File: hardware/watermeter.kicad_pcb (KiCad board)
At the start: 2 copper layers, 80 x 40 mm, 46 parts, among them J1 TC2030, J2 EXT, J3 flow_meter, J4 PT1000-1, J5 PT1000-2, J6 24V_Power, SW1 Reboot, U1 ESP32-C6-MINI-1, U2 TLV2462AID, U3 K7805-500R3, U4 LM3671MFX-3.3/NOPB

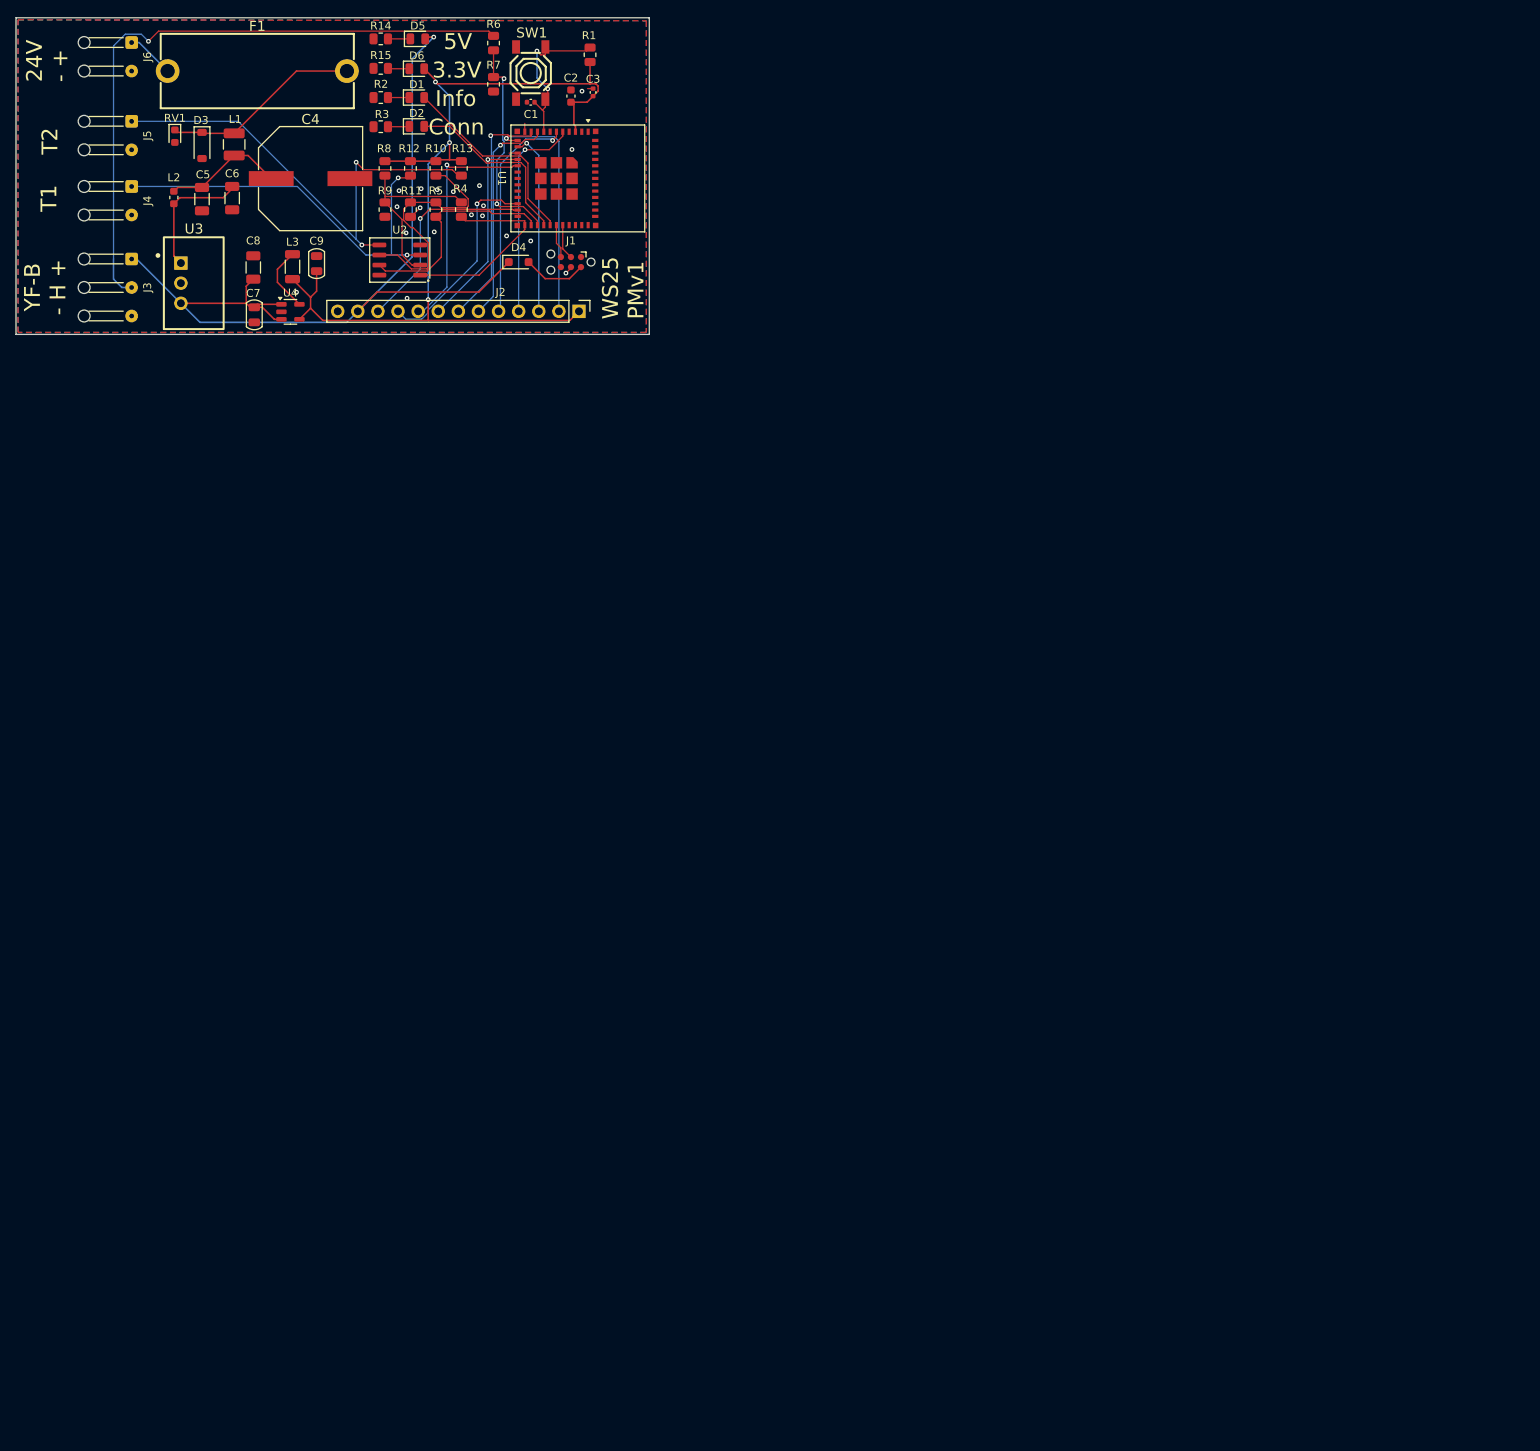
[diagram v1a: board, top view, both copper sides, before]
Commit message: Release hardware design v1.0 for manufacturing
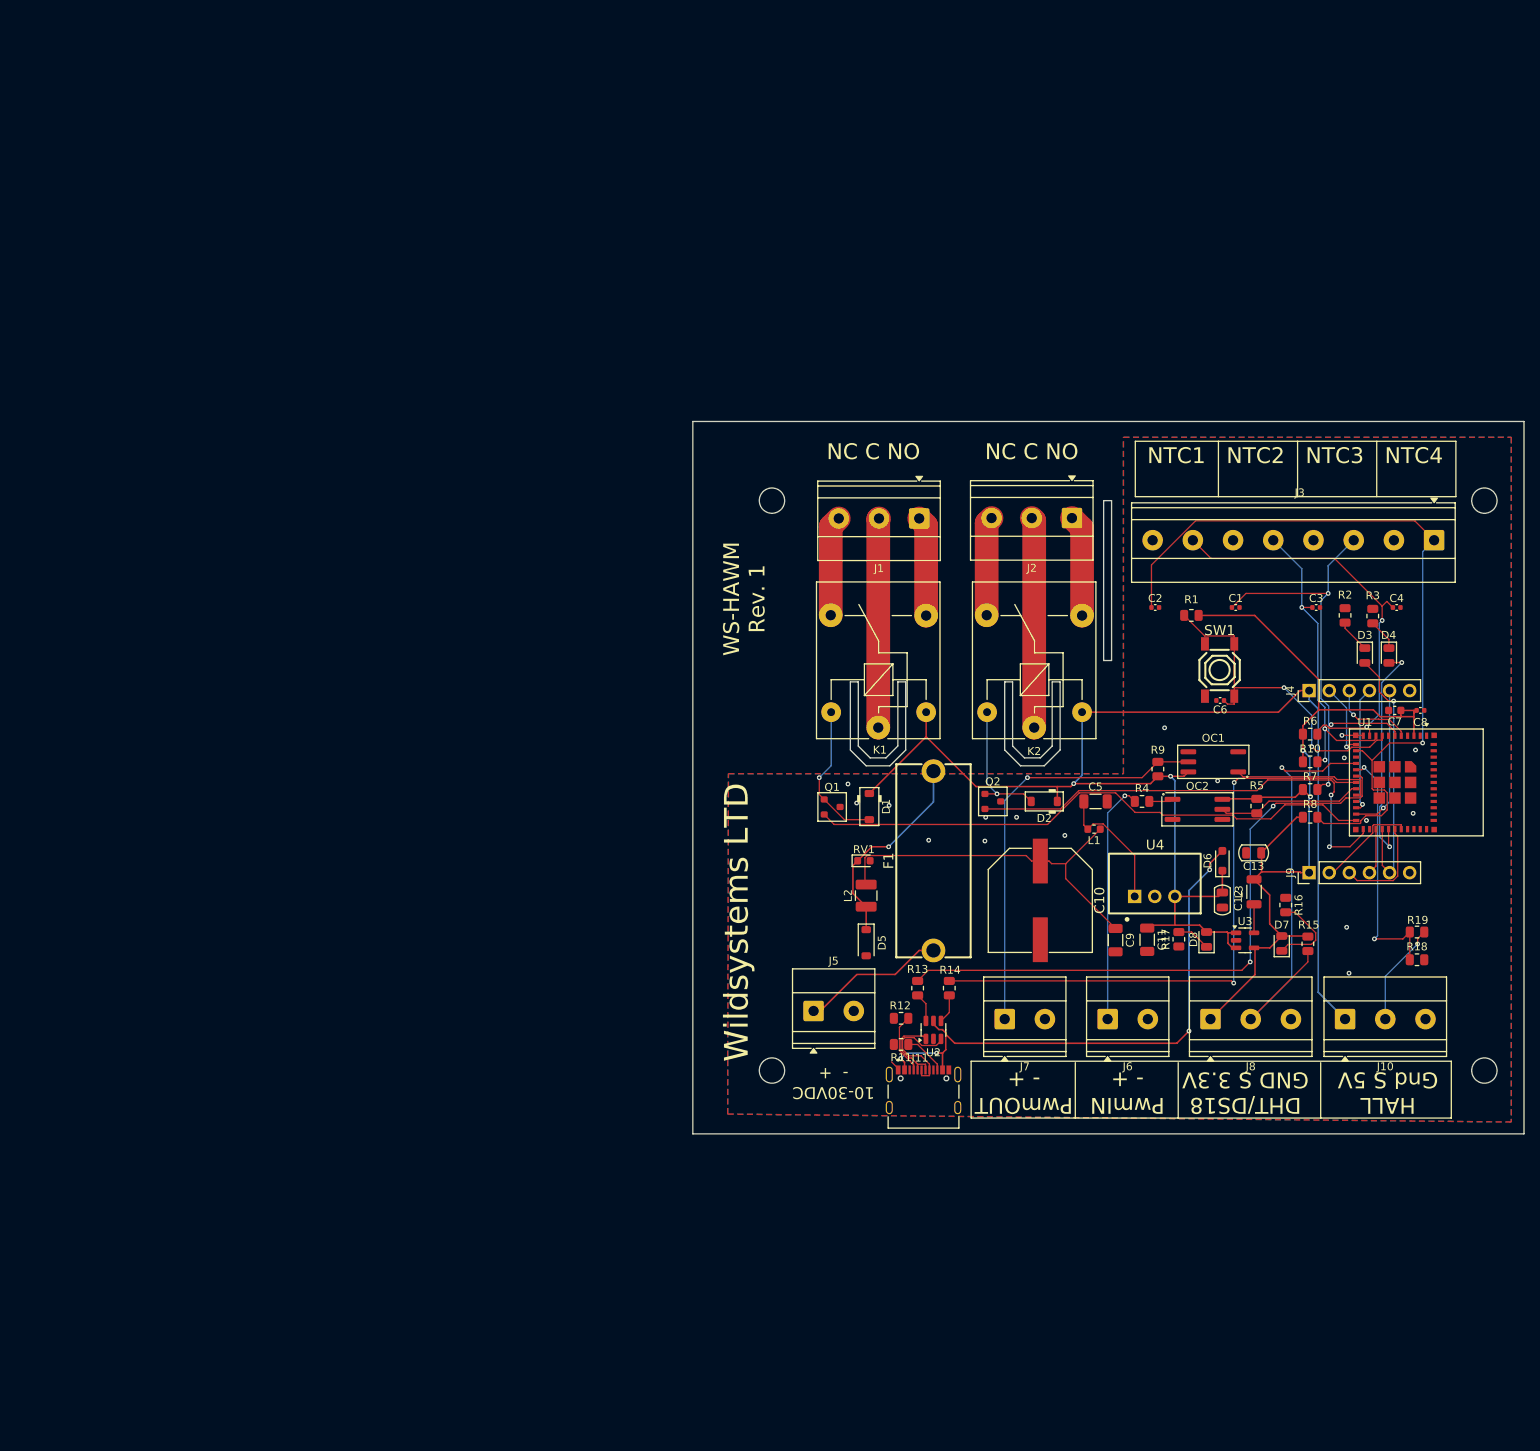
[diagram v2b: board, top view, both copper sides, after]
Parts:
- added C10: 680uF/50V, MyFootprints:CAP-SMD_BD12.5-L13.0-W13.0-LS14.4-FD, F.Cu at (129.4, 111.5)
- added C11: 22uF/10V, Capacitor_SMD:C_1206_3216Metric, F.Cu at (142.9, 116.5)
- added C12: 4.7uF/10V, PCM_Capacitor_SMD_AKL:C_0805_2012Metric, F.Cu at (152.4, 111.5)
- added C13: 10uF, PCM_Capacitor_SMD_AKL:C_0805_2012Metric, F.Cu at (156.3, 105.5)
- added D7: KT-0805G, LED_SMD:LED_0805_2012Metric, F.Cu at (159.9, 116.9)
- added D8: KT-0805G, LED_SMD:LED_0805_2012Metric, F.Cu at (150.4, 116.4)
- added H1: MountingHole, MountingHole:MountingHole_3.2mm_M3_ISO7380, F.Cu at (95.5, 61.0)
- added H2: MountingHole, MountingHole:MountingHole_3.2mm_M3_ISO7380, F.Cu at (185.5, 61.0)
- added H3: MountingHole, MountingHole:MountingHole_3.2mm_M3_ISO7380, F.Cu at (95.5, 133.0)
- added H4: MountingHole, MountingHole:MountingHole_3.2mm_M3_ISO7380, F.Cu at (185.5, 133.0)
- added J10: flow_meter, TerminalBlock_Phoenix:TerminalBlock_Phoenix_MKDS-1,5-3-5.08_1x03_P5.08mm_Horizontal, F.Cu at (167.9, 126.5)
- added J11: USB-TYPE-C-31-M-12, MyFootprints:USB-HRO_TYPE-C-31-M-12, F.Cu at (114.6, 137.7)
- added J7: PWM_OUT, TerminalBlock_Phoenix:TerminalBlock_Phoenix_MKDS-1,5-2-5.08_1x02_P5.08mm_Horizontal, F.Cu at (124.9, 126.5)
- added J8: DHT21, TerminalBlock_Phoenix:TerminalBlock_Phoenix_MKDS-1,5-3-5.08_1x03_P5.08mm_Horizontal, F.Cu at (150.9, 126.5)
- added J9: Conn_01x06_Shielded, Connector_PinHeader_2.54mm:PinHeader_1x06_P2.54mm_Vertical, F.Cu at (163.4, 108.0)
- added K1: SRD-05VDC-SL-C, Relay_THT:Relay_SPDT_SANYOU_SRD_Series_Form_C, F.Cu at (108.9, 89.7)
- added K2: SRD-05VDC-SL-C, Relay_THT:Relay_SPDT_SANYOU_SRD_Series_Form_C, F.Cu at (128.6, 89.7)
- added OC1: TLP2361, PCM_Package_SO_AKL:SO-5_4.4x3.6mm_P1.27mm, F.Cu at (151.2, 94.0)
- added OC2: TLP2361, PCM_Package_SO_AKL:SO-5_4.4x3.6mm_P1.27mm, F.Cu at (149.2, 100.0)
- added Q1: NPN, PCM_Package_TO_SOT_SMD_AKL:SOT-23, F.Cu at (103.1, 99.7)
- added Q2: NPN, PCM_Package_TO_SOT_SMD_AKL:SOT-23, F.Cu at (123.4, 99.0)
- added R16: 20R, Resistor_SMD:R_0805_2012Metric, F.Cu at (160.4, 112.1)
- added R17: 20R, Resistor_SMD:R_0805_2012Metric, F.Cu at (146.9, 116.4)
- added R18: 2k, Resistor_SMD:R_0805_2012Metric, F.Cu at (177.0, 119.0)
- added R19: 1k, Resistor_SMD:R_0805_2012Metric, F.Cu at (177.0, 115.5)
- C1: value 1uF -> 0.1uF
- C2: value 22uF -> 0.1uF; footprint Capacitor_SMD:C_0603_1608Metric -> Capacitor_SMD:C_0402_1005Metric
- C4: value 680uF/50V -> 0.1uF; footprint MyFootprints:CAP-SMD_BD12.5-L13.0-W13.0-LS14.4-FD -> Capacitor_SMD:C_0402_1005Metric
- C5: value 4.7uF/63V -> 10uF/50V
- C6: value 10uF/50V -> 1uF; footprint Capacitor_SMD:C_1206_3216Metric -> Capacitor_SMD:C_0402_1005Metric
- C7: value 4.7uF/10V -> 22uF; footprint PCM_Capacitor_SMD_AKL:C_0805_2012Metric -> Capacitor_SMD:C_0603_1608Metric
- C8: value 22uF/10V -> 0.1uF; footprint Capacitor_SMD:C_1206_3216Metric -> Capacitor_SMD:C_0402_1005Metric
- C9: value 10uF -> 4.7uF/63V; footprint PCM_Capacitor_SMD_AKL:C_0805_2012Metric -> Capacitor_SMD:C_1206_3216Metric
- D1: value KT-0805G -> 1N4148W; footprint LED_SMD:LED_0805_2012Metric -> PCM_Diode_SMD_AKL:D_SOD-123
- D2: value KT-0805B -> 1N4148W; footprint Diode_SMD:D_0805_2012Metric -> PCM_Diode_SMD_AKL:D_SOD-123
- D3: value BAT46W -> KT-0805B; footprint Diode_SMD:D_SOD-123 -> Diode_SMD:D_0805_2012Metric
- D4: value 1N5819 -> KT-0805G; footprint Diode_SMD:D_SOD-323_HandSoldering -> LED_SMD:LED_0805_2012Metric
- D5: value KT-0805G -> BAT46W; footprint LED_SMD:LED_0805_2012Metric -> Diode_SMD:D_SOD-123
- D6: value KT-0805G -> 1N5819; footprint LED_SMD:LED_0805_2012Metric -> Diode_SMD:D_SOD-323_HandSoldering
- J1: value TC2030 -> Screw_Terminal_01x03; footprint Connector:Tag-Connect_TC2030-IDC-NL_2x03_P1.27mm_Vertical -> TerminalBlock_Phoenix:TerminalBlock_Phoenix_MKDS-1,5-3-5.08_1x03_P5.08mm_Horizontal
- J2: value EXT -> Screw_Terminal_01x03; footprint Connector_PinHeader_2.54mm:PinHeader_1x13_P2.54mm_Vertical -> TerminalBlock_Phoenix:TerminalBlock_Phoenix_MKDS-1,5-3-5.08_1x03_P5.08mm_Horizontal
- J3: value flow_meter -> Conn_01x08_Pin; footprint Connector_Wire:SolderWire-0.1sqmm_1x03_P3.6mm_D0.4mm_OD1mm_Relief -> TerminalBlock_Phoenix:TerminalBlock_Phoenix_MKDS-1,5-8-5.08_1x08_P5.08mm_Horizontal
- J4: value PT1000-1 -> Conn_01x06_Shielded; footprint Connector_Wire:SolderWire-0.1sqmm_1x02_P3.6mm_D0.4mm_OD1mm_Relief -> Connector_PinHeader_2.54mm:PinHeader_1x06_P2.54mm_Vertical
- J5: value PT1000-2 -> 24V_Power; footprint Connector_Wire:SolderWire-0.1sqmm_1x02_P3.6mm_D0.4mm_OD1mm_Relief -> TerminalBlock_Phoenix:TerminalBlock_Phoenix_MKDS-1,5-2-5.08_1x02_P5.08mm_Horizontal
- J6: value 24V_Power -> PWM_IN; footprint Connector_Wire:SolderWire-0.1sqmm_1x02_P3.6mm_D0.4mm_OD1mm_Relief -> TerminalBlock_Phoenix:TerminalBlock_Phoenix_MKDS-1,5-2-5.08_1x02_P5.08mm_Horizontal
- L1: value FHW1210IF820JST -> 22uH; footprint Inductor_SMD:L_1210_3225Metric -> Inductor_SMD:L_0603_1608Metric
- L2: value 22uH -> FHW1210IF820JST; footprint Inductor_SMD:L_0603_1608Metric -> Inductor_SMD:L_1210_3225Metric
- R11: value 1k -> 5k1
- R12: value 4k7 -> 5k1
- R13: value 4k7 -> 22R
- R14: value 20R -> 22R
- R15: value 20R -> 10K
- R2: value 20R -> 15R
- R3: value 15R -> 20R
- R4: value 20k -> 1k
- R5: value 20k -> 4k7
- R6, R9: value 1k -> 4k7
- R7: value 2k -> 4k7
- U2: value TLV2462AID -> USBLC6-2SC6; footprint PCM_Package_SO_AKL:SO-8_3.9x4.9mm_P1.27mm -> Package_TO_SOT_SMD:SOT-23-6
- U3: value K7805-500R3 -> LM3671MFX-3.3/NOPB; footprint MyFootprints:PWRM-TH_K78XX-500R3 -> Package_TO_SOT_SMD:TSOT-23-5
- U4: value LM3671MFX-3.3/NOPB -> K7805-500R3; footprint Package_TO_SOT_SMD:TSOT-23-5 -> MyFootprints:PWRM-TH_K78XX-500R3
- moved J6 174.4 mm to (137.9, 126.5), turned to 0 degrees
- moved J3 168.3 mm to (179.2, 66.0), turned to 180 degrees
- moved J4 161.8 mm to (163.4, 85.0), turned to 90 degrees
- moved R15 161.1 mm to (163.2, 117.0), turned to -90 degrees
- moved D3 160.4 mm to (170.4, 80.6)
- moved U3 158.0 mm to (155.3, 116.5), turned to 0 degrees
- moved C8 157.7 mm to (177.4, 87.5), turned to 0 degrees
- moved C7 152.5 mm to (174.2, 87.5), turned to 180 degrees
- moved C4 147.5 mm to (174.4, 74.5)
- moved L3 144.9 mm to (156.4, 110.4), turned to 90 degrees
- moved R8 142.8 mm to (163.5, 101.0), turned to 0 degrees
- moved D6 142.7 mm to (152.4, 106.5), turned to 90 degrees
- moved J5 141.6 mm to (100.8, 125.5), turned to 0 degrees
- moved C6 140.0 mm to (152.1, 86.2), turned to 180 degrees
- moved R14 139.8 mm to (117.9, 122.6), turned to 90 degrees
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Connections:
- C1 pad 1: Net-(U1-EN) -> /IO3
- C2 pad 1: +3.3V -> /IO1
- C3 pad 1: +3.3V -> /IO4
- C4 pad 1: Net-(C4-Pad1) -> /IO5
- C5 pad 1: Net-(C4-Pad1) -> Net-(U4-IN)
- C6 pad 1: Net-(U3-IN) -> Net-(U1-EN)
- C7 pad 1: +5V -> +3.3V
- C8 pad 1: +5V -> +3.3V
- C9 pad 1: +3.3V -> Net-(C10-Pad1)
- D1 pad 1: Net-(D1-K) -> +5V
- D2 pad 1: Net-(D2-K) -> +5V
- D3 pad 1: /24V_FUSED -> Net-(D3-K)
- D3 pad 2: GND -> /IO22
- D4 pad 1: +5V -> Net-(D4-K)
- D4 pad 2: /5V_USB -> /IO23
- D5 pad 1: Net-(D5-K) -> /24V_FUSED
- D5 pad 2: +5V -> GND
- D6 pad 1: Net-(D6-K) -> +5V
- D6 pad 2: +3.3V -> /5V_USB
- J1 pad 1: /EN -> /NO1
- J1 pad 2: /5V_USB -> /COM1
- J1 pad 3: /TXD -> /NC1
- J2 pad 1: +3.3V -> /NO2
- J2 pad 2: Net-(J2-Pin_2) -> /COM2
- J2 pad 3: Net-(J2-Pin_3) -> /NC2
- J3 pad 1: +5V -> /IO1
- J3 pad 2: Net-(J3-Pin_2) -> GND
- J3 pad 3: GND -> /IO3
- J4 pad 1: Net-(J4-Pin_1) -> +5V
- J4 pad 2: GND -> /IO0
- J5 pad 1: Net-(J5-Pin_1) -> /Power/24V
- J6 pad 1: /Power/24V -> Net-(J6-Pin_1)
- L1 pad 1: /24V_FUSED -> Net-(C10-Pad1)
- L1 pad 2: Net-(C4-Pad1) -> Net-(U4-IN)
- L2 pad 1: Net-(C4-Pad1) -> /24V_FUSED
- L2 pad 2: Net-(U3-IN) -> Net-(C10-Pad1)
- L3 pad 1: Net-(U4-SW) -> Net-(U3-SW)
- R10 pad 2: Net-(U2B--) -> /IO4
- R11 pad 1: Net-(U2B--) -> Net-(J11-CC2)
- R12 pad 1: +3.3V -> Net-(J11-CC1)
- R12 pad 2: Net-(J4-Pin_1) -> GND
- R13 pad 1: +3.3V -> Net-(R13-Pad1)
- R13 pad 2: Net-(J5-Pin_1) -> /USB_D_N
- R14 pad 1: GND -> Net-(R14-Pad1)
- R14 pad 2: Net-(D5-K) -> /USB_D_P
- R15 pad 1: GND -> +3.3V
- R15 pad 2: Net-(D6-K) -> /IO6
- R2 pad 1: Net-(D1-K) -> Net-(D3-K)
- R3 pad 1: Net-(D2-K) -> Net-(D4-K)
- R4 pad 1: Net-(U2A--) -> Net-(J6-Pin_1)
- R4 pad 2: Net-(U1-IO19) -> Net-(OC2-Pad1)
- R5 pad 1: Net-(U2B--) -> +3.3V
- R5 pad 2: Net-(U1-IO20) -> /IO14
- R6 pad 1: Net-(J3-Pin_2) -> +3.3V
- R6 pad 2: Net-(U1-IO21) -> /IO5
- R7 pad 1: Net-(U1-IO21) -> +3.3V
- R7 pad 2: GND -> /IO3
- R8 pad 2: Net-(U2A--) -> /IO1
- R9 pad 1: Net-(U2A--) -> +5V
- R9 pad 2: GND -> Net-(J7-Pin_1)
- U1 pad 10: Net-(J2-Pin_7) -> /IO5
- U1 pad 12: Net-(J2-Pin_2) -> /IO0
- U1 pad 13: Net-(J2-Pin_3) -> /IO1
- U1 pad 15: Net-(J2-Pin_8) -> /IO6
- U1 pad 16: Net-(J2-Pin_9) -> /IO7
- U1 pad 17: unconnected-(U1-IO12-Pad17) -> /USB_D_N
- U1 pad 18: unconnected-(U1-IO13-Pad18) -> /USB_D_P
- U1 pad 19: unconnected-(U1-IO14-Pad19) -> /IO14
- U1 pad 20: unconnected-(U1-IO15-Pad20) -> /IO15
- U1 pad 22: Net-(J2-Pin_10) -> /IO8
- U1 pad 23: Net-(J2-Pin_11) -> /IO9
- U1 pad 24: unconnected-(U1-IO18-Pad24) -> /IO18
- U1 pad 25: Net-(U1-IO19) -> /IO19
- U1 pad 26: Net-(U1-IO20) -> /IO20
- U1 pad 27: Net-(U1-IO21) -> /IO21
- U1 pad 28: Net-(D2-A) -> /IO22
- U1 pad 29: Net-(D1-A) -> /IO23
- U1 pad 30: /RXD -> /RXD0
- U1 pad 31: /TXD -> /TXD0
- U1 pad 5: Net-(J2-Pin_4) -> /IO2
- U1 pad 6: Net-(J2-Pin_5) -> /IO3
- U1 pad 9: Net-(J2-Pin_6) -> /IO4
- U2 pad 1: Net-(U1-IO19) -> /D-
- U2 pad 2: Net-(U2A--) -> GND
- U2 pad 3: Net-(J4-Pin_1) -> /D+
- U2 pad 4: unconnected-(U2A-V--Pad4) -> Net-(R14-Pad1)
- U2 pad 5: Net-(J5-Pin_1) -> /5V_USB
- U2 pad 6: Net-(U2B--) -> Net-(R13-Pad1)
- U3 pad 1: Net-(U3-IN) -> +5V
- U4 pad 1: +5V -> Net-(U4-IN)
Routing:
- net /IO1: track 0.00 -> 98.3 mm, vias 0 -> 1
- net Net-(J3-Pin_2): track 82.0 -> 0.00 mm, vias 1 -> 0
- net /USB_D_N: track 0.00 -> 78.8 mm, vias 0 -> 2
- net /USB_D_P: track 0.00 -> 77.2 mm, vias 0 -> 2
- net /IO18: track 0.00 -> 72.3 mm
- net /5V_USB: track 8.10 -> 70.8 mm, vias 0 -> 4
- net +5V: track 114.5 -> 176.6 mm, vias 1 -> 2
- net Net-(J5-Pin_1): track 61.5 -> 0.00 mm, vias 2 -> 0
- net /IO19: track 0.00 -> 59.6 mm, vias 0 -> 2
- net /IO3: track 0.00 -> 56.9 mm, vias 0 -> 3
- net /IO6: track 0.00 -> 56.0 mm, vias 0 -> 1
- net /IO5: track 0.00 -> 53.8 mm, vias 0 -> 2
- net Net-(J7-Pin_1): track 0.00 -> 52.8 mm, vias 0 -> 1
- net Net-(J4-Pin_1): track 51.8 -> 0.00 mm, vias 2 -> 0
- net Net-(C10-Pad1): track 0.00 -> 46.3 mm
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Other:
- board size 80 x 40 mm -> 105 x 90 mm
- board text added: "+3.3v TXD0 RXD0 IO21 IO22 GND"
- board text added: "+5V IO0 IO2 IO8 IO9 GND"
- board text added: "10-30VDC - +"
- board text added: "DHT/DS18 GND S 3.3V"
- board text added: "HALL Gnd S 5V"
- board text added: "NC C NO"
- board text added: "NTC1"
- board text added: "NTC2"
- board text added: "NTC3"
- board text added: "NTC4"
- board text added: "Pin Function IO0 EXT_IO0 IO1 EXT_IO1 IO2 EXT_IO2 IO3 DHT21/DS18 IO4 NTC1 IO5 FLOW IO6 PWM_IN IO7 NTC2 IO8 PWM_OUT IO9 EXT_IO9 IO18 RELAY1 IO19 RELAY2 IO22 LED1 IO23 LED2"
- board text added: "PwmIN - +"
- board text added: "PwmOUT - +"
- board text added: "WS-HAWM Rev. 1"
- board text added: "Wildsystems LTD"
- board text removed: "24V - +"
- board text removed: "3.3V"
- board text removed: "5V"
- board text removed: "Conn"
- board text removed: "Info"
- board text removed: "T1"
- board text removed: "T2"
- board text removed: "WS25 PMv1"
- board text removed: "YF-B - H +"
